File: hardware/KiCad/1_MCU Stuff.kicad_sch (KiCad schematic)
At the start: 16 parts, among them U1 STM32F072RBT6

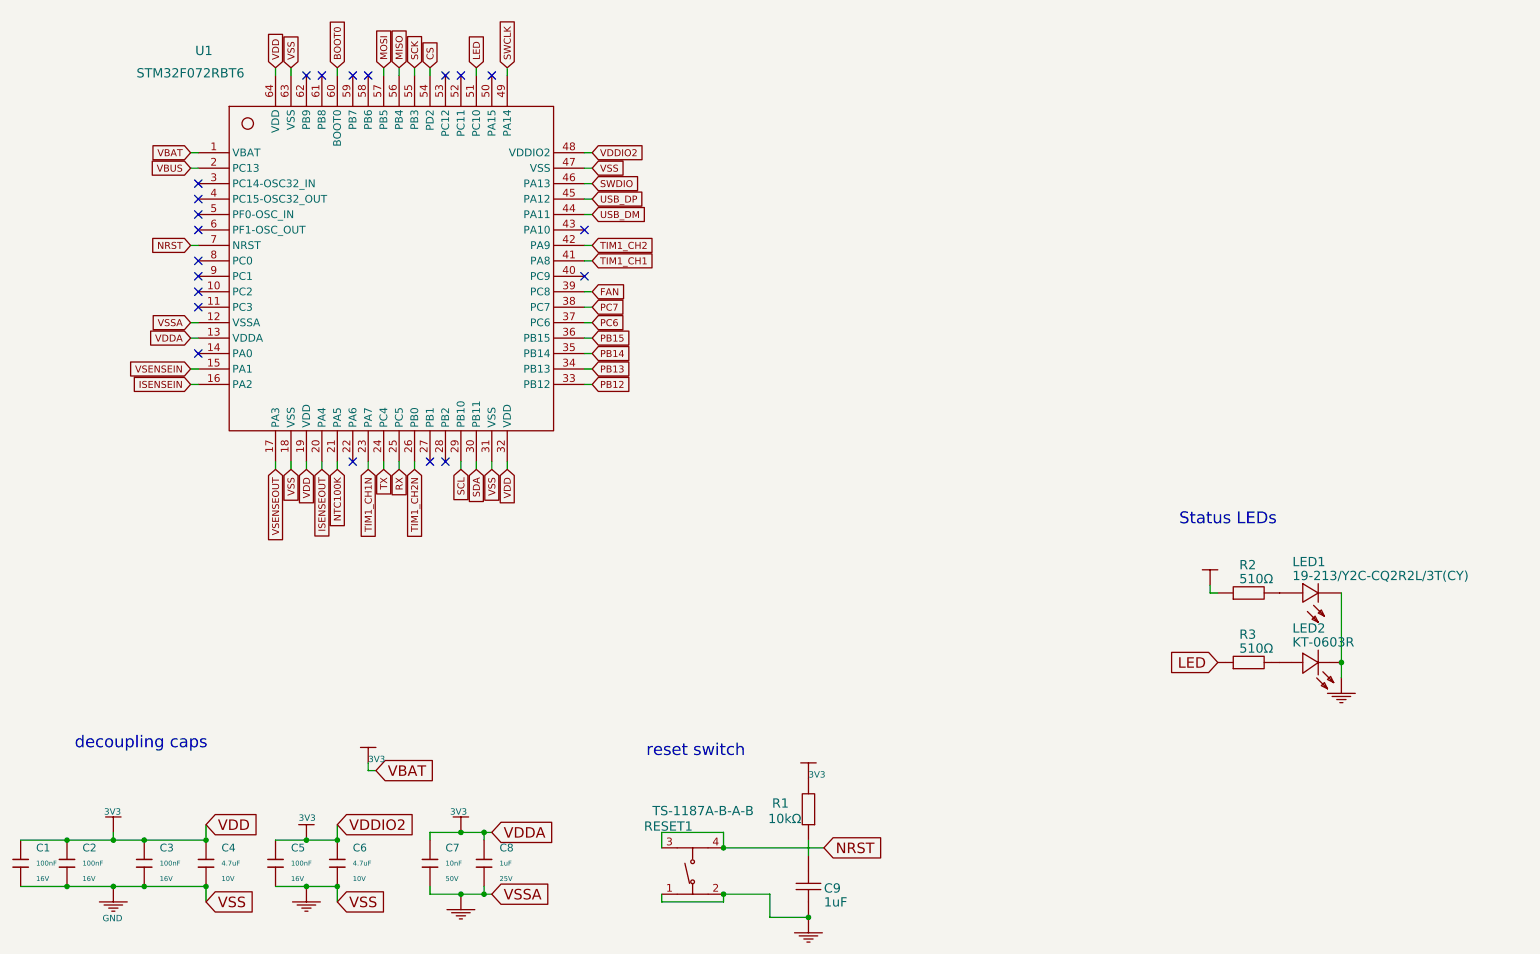
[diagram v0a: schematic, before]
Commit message: updates
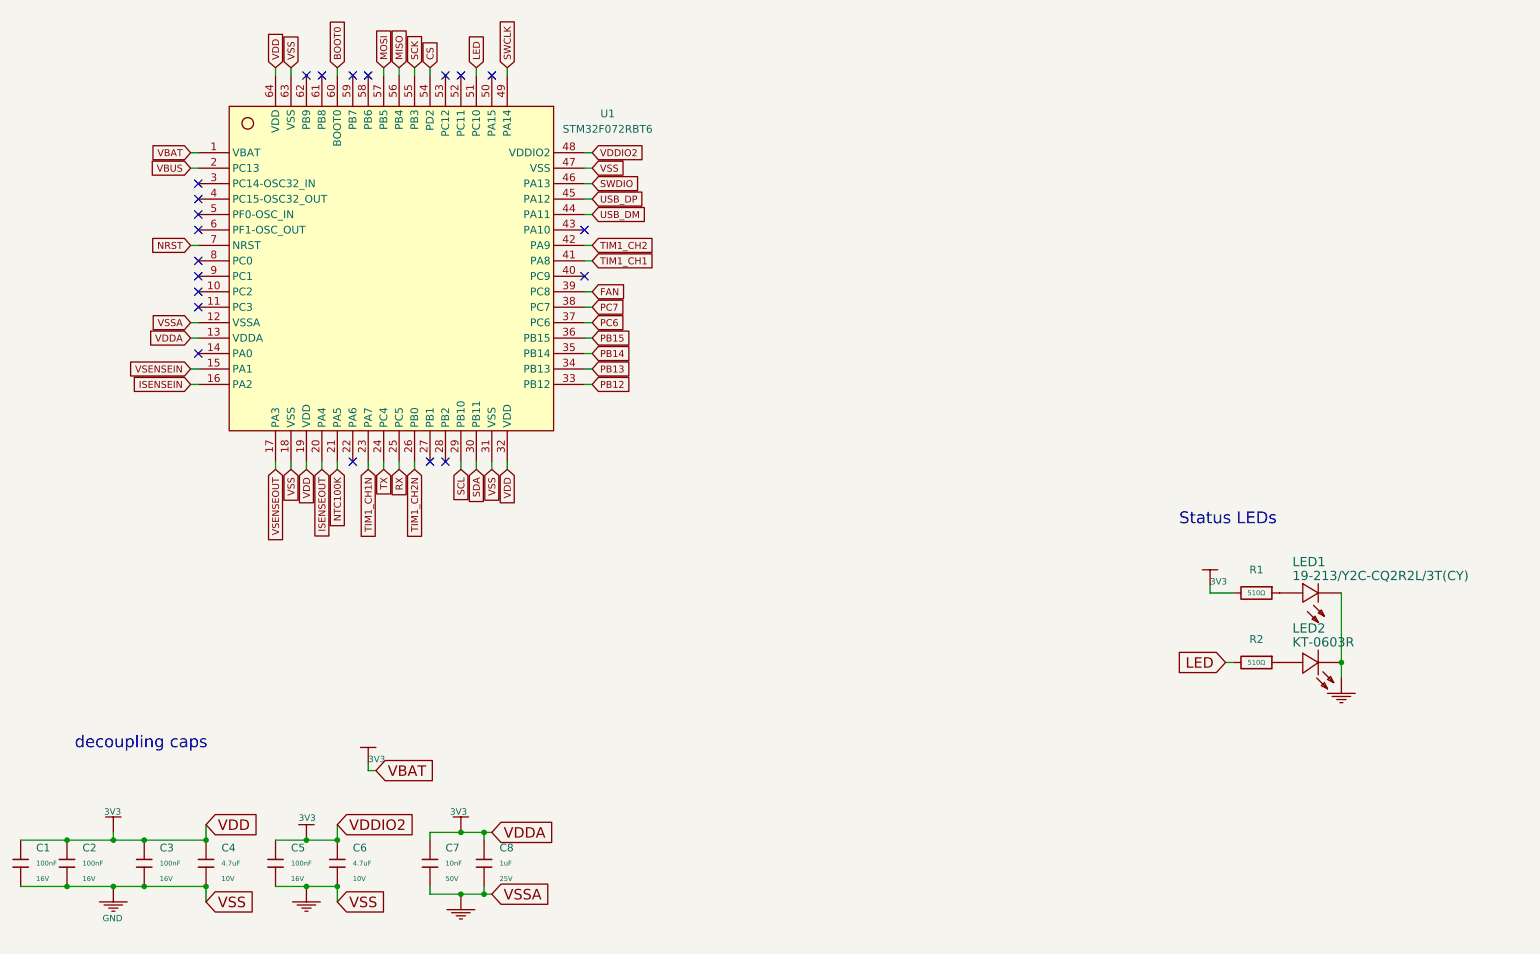
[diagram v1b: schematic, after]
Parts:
- removed C9: 1uF, ProPrj_STM-easyedapro:C0402, symbol ProPrj_STM-easyedapro:1uF
- removed R1: 10kΩ, ProPrj_STM-easyedapro:R0402, symbol ProPrj_STM-easyedapro:10kΩ
- removed R2, R3: 510Ω, ProPrj_STM-easyedapro:R0603, symbol ProPrj_STM-easyedapro:510Ω
- removed RESET1: TS-1187A-B-A-B, ProPrj_STM-easyedapro:SW-SMD_4P-L5.1-W5.1-P3.70-LS6.5-TL-2, symbol ProPrj_STM-easyedapro:TS-1187A-B-A-B
- removed U1: STM32F072RBT6, ProPrj_STM-easyedapro:LQFP-64_L10.0-W10.0-P0.50-LS12.0-BL, symbol ProPrj_STM-easyedapro:STM32F072RBT6
- added R1, R2: 510Ω, PCM_JLCPCB:R_0402, symbol JLCPCB-Resistors:0402,510Ω
- added U1: STM32F072RBT6, easyeda2kicad:LQFP-64_L10.0-W10.0-P0.50-LS12.0-BL, symbol easyeda2kicad:STM32F072RBT6
- LED1: footprint ProPrj_STM-easyedapro:LED0603-RD-YELLOW -> LED_SMD:LED_0603_1608Metric
- LED2: footprint ProPrj_STM-easyedapro:LED0603-RD -> LED_SMD:LED_0603_1608Metric
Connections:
- net 3V3: now also R1.2, U1.1 (VBAT), U1.13 (VDDA), U1.19 (VDD), U1.32 (VDD), U1.48 (VDDIO2), U1.64 (VDD)
- net BOOT0: now also U1.60 (BOOT0)
- net CS: now also U1.54 (PD2)
- net FAN: now also U1.39 (PC8)
- net GND: now also U1.12 (VSSA), U1.18 (VSS), U1.31 (VSS), U1.47 (VSS), U1.63 (VSS)
- net ISENSEIN: now also U1.16 (PA2)
- net ISENSEOUT: now also U1.20 (PA4)
- net LED: now also R2.2, U1.51 (PC10)
- net MISO: now also U1.56 (PB4)
- net MOSI: now also U1.57 (PB5)
- net NRST: now also U1.7 (NRST)
- net NTC100K: now also U1.21 (PA5)
- net PB12: now also U1.33 (PB12)
- net PB13: now also U1.34 (PB13)
- net PB14: now also U1.35 (PB14)
- net PB15: now also U1.36 (PB15)
- net PC6: now also U1.37 (PC6)
- net PC7: now also U1.38 (PC7)
- net RX: now also U1.25 (PC5)
- net SCK: now also U1.55 (PB3)
- net SCL: now also U1.29 (PB10)
- net SDA: now also U1.30 (PB11)
- net SWCLK: now also U1.49 (PA14)
- net SWDIO: now also U1.46 (PA13)
- net TIM1_CH1: now also U1.41 (PA8)
- net TIM1_CH1N: now also U1.23 (PA7)
- net TIM1_CH2: now also U1.42 (PA9)
- net TIM1_CH2N: now also U1.26 (PB0)
- net TX: now also U1.24 (PC4)
- net USB_DM: now also U1.44 (PA11)
- net USB_DP: now also U1.45 (PA12)
- net VBUS: now also U1.2 (PC13)
- net VSENSEIN: now also U1.15 (PA1)
- net VSENSEOUT: now also U1.17 (PA3)
- net at LED1.2 (A): now also R1.1
- net at LED2.2 (A): now also R2.1
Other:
- note removed: "reset switch"
